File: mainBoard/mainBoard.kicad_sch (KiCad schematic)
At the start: 17 parts, among them J1 Conn_01x04, J2 Conn_01x04, J6 Conn_01x07, J7 Conn_01x07

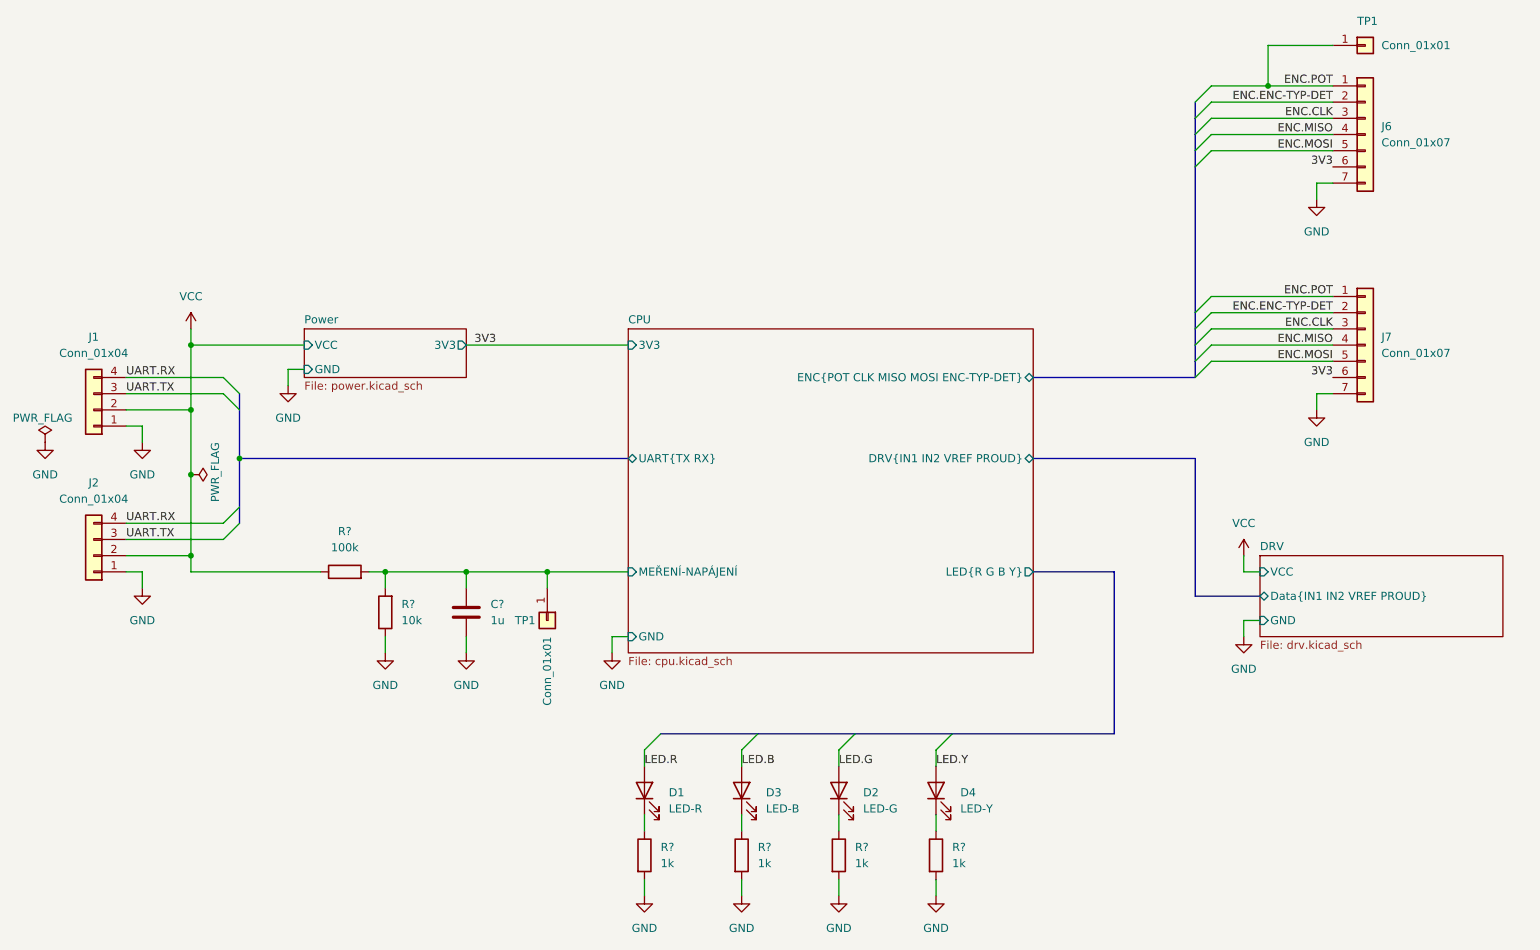
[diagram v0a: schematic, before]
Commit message: drobeček
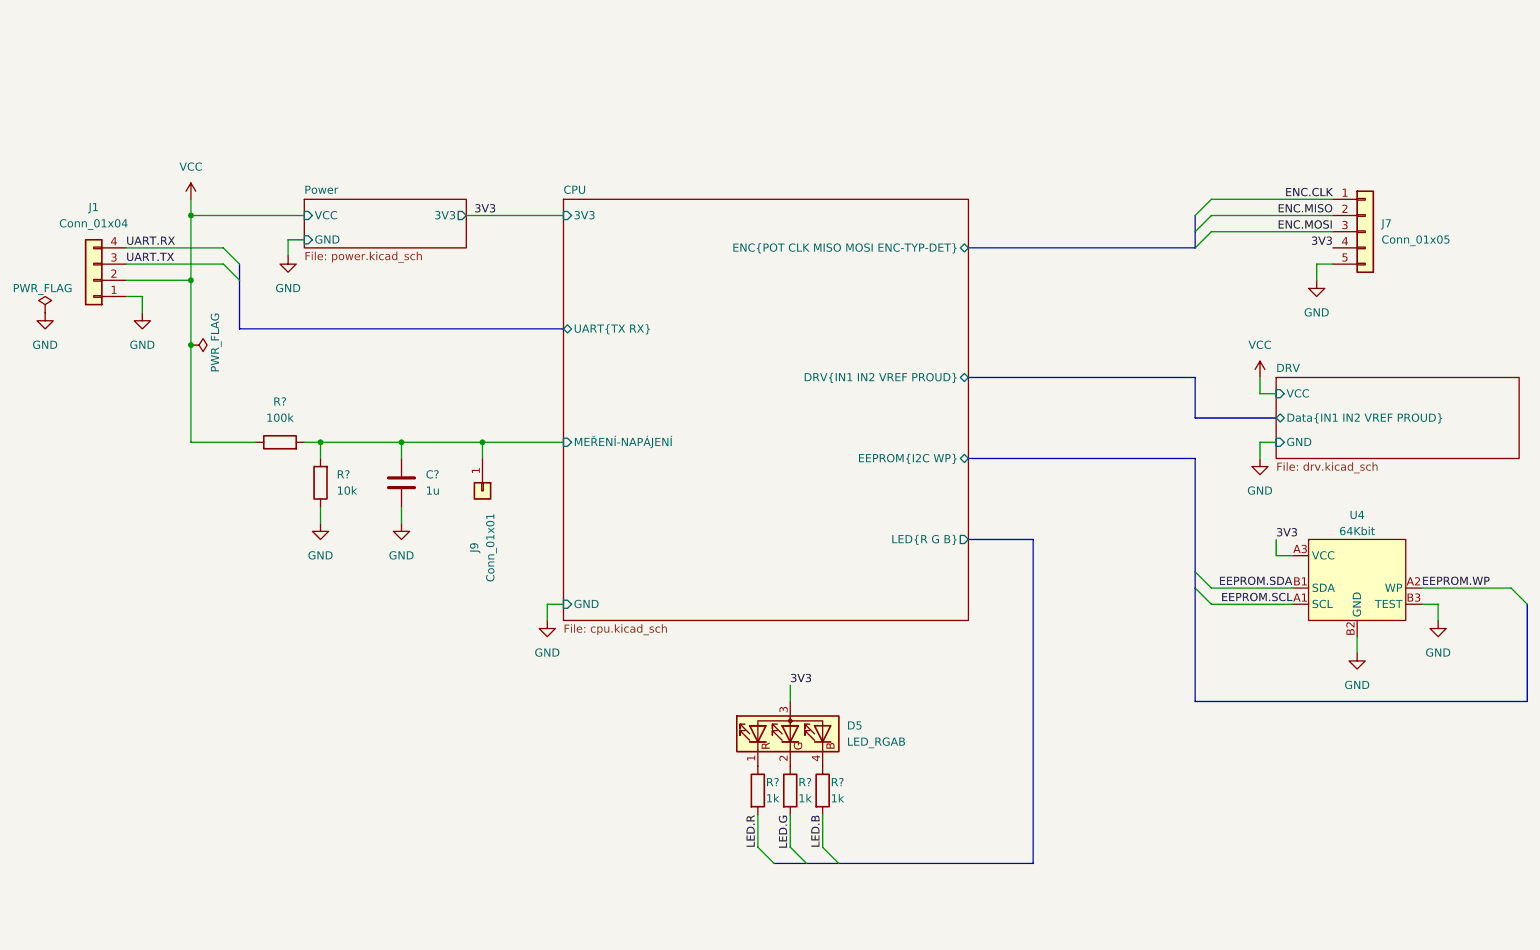
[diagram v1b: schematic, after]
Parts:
- removed D1: LED-R, LED_SMD:LED_0603_1608Metric, symbol Device:LED
- removed D2: LED-G, LED_SMD:LED_0603_1608Metric, symbol Device:LED
- removed D3: LED-B, LED_SMD:LED_0603_1608Metric, symbol Device:LED
- removed D4: LED-Y, LED_SMD:LED_0603_1608Metric, symbol Device:LED
- removed J2: Conn_01x04, Connector_JST:JST_PH_B4B-PH-K_1x04_P2.00mm_Vertical, symbol Connector_Generic:Conn_01x04
- removed J6: Conn_01x07, Connector_JST:JST_PH_B7B-PH-K_1x07_P2.00mm_Vertical, symbol Connector_Generic:Conn_01x07
- removed J7: Conn_01x07, Connector_PinHeader_1.27mm:PinHeader_1x07_P1.27mm_Vertical, symbol Connector_Generic:Conn_01x07
- removed R?: 1k, Capacitor_SMD:C_0402_1005Metric, symbol Device:R
- removed TP1 (x2): Conn_01x01, Connector_Pin:Pin_D1.0mm_L10.0mm, symbol Connector_Generic:Conn_01x01
- added D5: LED_RGAB, LED_SMD:LED_LiteOn_LTST-C19HE1WT, symbol Device:LED_RGAB
- added J7: Conn_01x05, Connector_PinHeader_2.00mm:PinHeader_1x05_P2.00mm_Vertical, symbol Connector_Generic:Conn_01x05
- added J9: Conn_01x01, RKL-Connectors:YZ157015035P-01-contact_pad, symbol Connector_Generic:Conn_01x01
- added U4: 64Kbit, RKL-StandardPackages:XFBGA-6, symbol RKL-Memory:BRCC064GWZ-3E2
- R?: footprint Capacitor_SMD:C_0402_1005Metric -> Resistor_SMD:R_0201_0603Metric; LCSC C25744 -> C473048
- R? (x3): footprint Capacitor_SMD:C_0402_1005Metric -> Capacitor_SMD:C_0201_0603Metric; LCSC C852624 -> C138165
- R?: footprint Capacitor_SMD:C_0402_1005Metric -> Resistor_SMD:R_0201_0603Metric; LCSC C25741 -> C320497
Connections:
- net 3V3: now also D5.3 (A), J7.4 (Pin_4), U4.A3 (VCC)
- net CPU/MEŘENÍ-NAPÁJENÍ: now also J9.1 (Pin_1)
- net ENC.CLK: now also J7.1 (Pin_1)
- net ENC.MISO: now also J7.2 (Pin_2)
- net ENC.MOSI: now also J7.3 (Pin_3)
- net GND: now also J7.5 (Pin_5), U4.B2 (GND), U4.B3 (TEST); no longer R?.2, R?.2, R?.2
- net LED.B: now also R?.2
- net LED.G: now also R?.2
- net LED.R: now also R?.2
- net at R?.1: now also D5.1 (RK)
- net at R?.1: now also D5.4 (BK)
- net at R?.1: now also D5.2 (GK)
- new net EEPROM.SCL: U4.A1 (SCL)
- new net EEPROM.SDA: U4.B1 (SDA)
- new net EEPROM.WP: U4.A2 (WP)
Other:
- sheet CPU ports: added EEPROM{I2C WP}, LED{R G B}; removed LED{R G B Y}
- moved on the sheet: C?, J1, R?

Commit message: Wpi
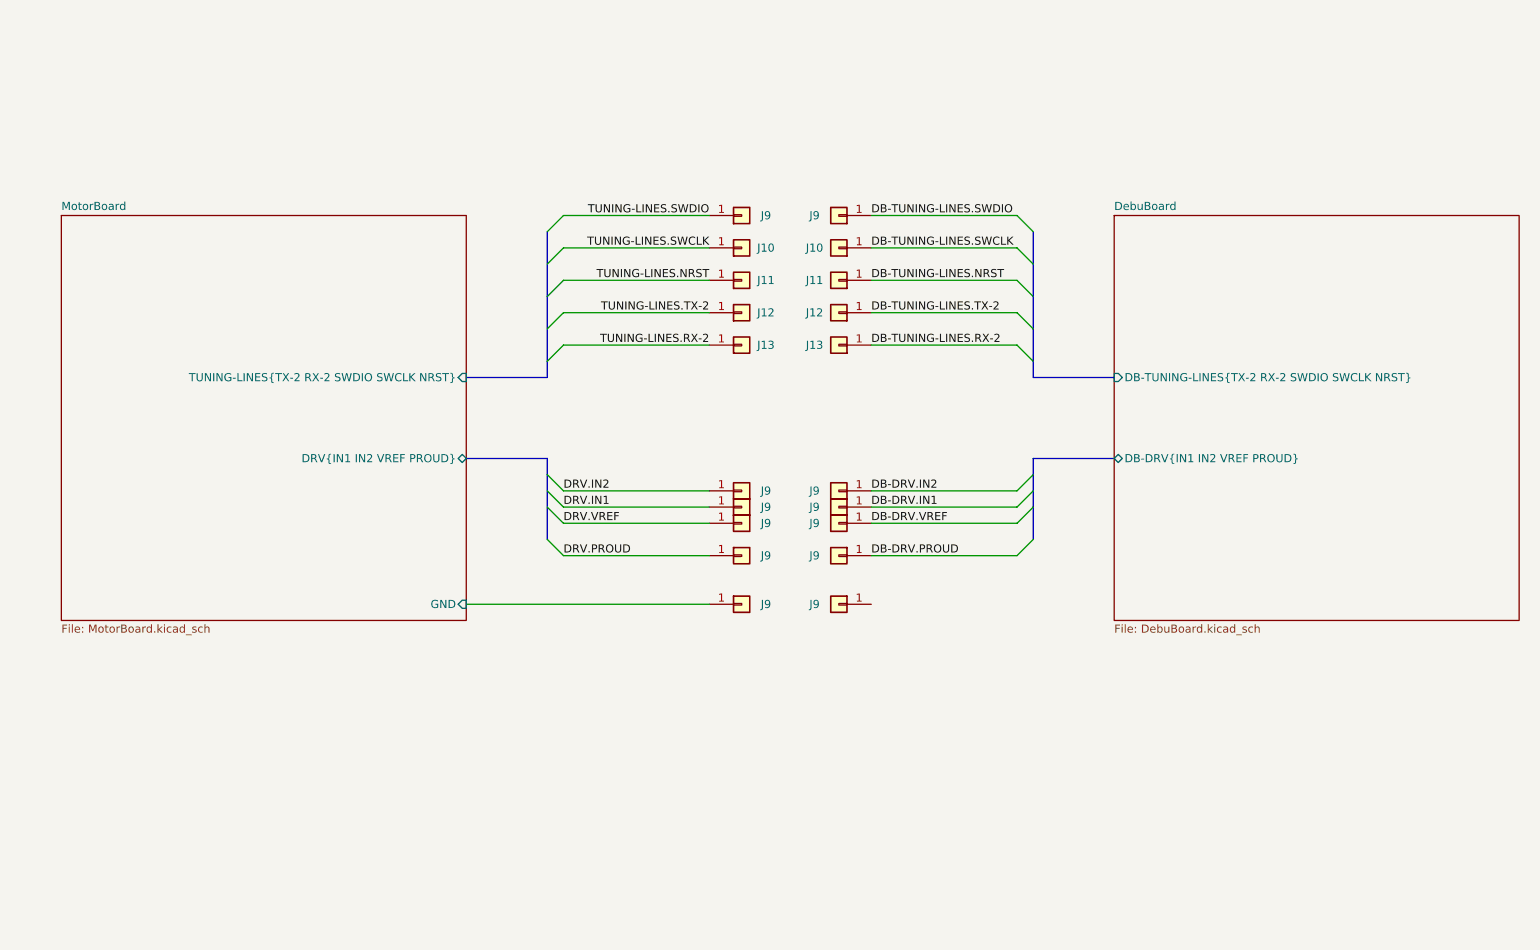
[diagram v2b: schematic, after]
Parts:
- removed C?: 1u, Capacitor_SMD:C_0402_1005Metric, symbol Device:C
- removed D5: LED_RGAB, LED_SMD:LED_LiteOn_LTST-C19HE1WT, symbol Device:LED_RGAB
- removed J1: Conn_01x04, Connector_JST:JST_PH_B4B-PH-K_1x04_P2.00mm_Vertical, symbol Connector_Generic:Conn_01x04
- removed J7: Conn_01x05, Connector_PinHeader_2.00mm:PinHeader_1x05_P2.00mm_Vertical, symbol Connector_Generic:Conn_01x05
- removed J9: Conn_01x01, RKL-Connectors:YZ157015035P-01-contact_pad, symbol Connector_Generic:Conn_01x01
- removed R?: 10k, Resistor_SMD:R_0201_0603Metric, symbol Device:R
- removed R? (x3): 1k, Capacitor_SMD:C_0201_0603Metric, symbol Device:R
- removed R?: 100k, Resistor_SMD:R_0201_0603Metric, symbol Device:R
- removed U4: 64Kbit, RKL-StandardPackages:XFBGA-6, symbol RKL-Memory:BRCC064GWZ-3E2
- added J10, J11, J12, J13, J9 (x6): Conn_01x01, RKL-Connectors:YZ157015035P-01, symbol Connector_Generic:Conn_01x01
- added J10, J11, J12, J13, J9 (x6): Conn_01x01, RKL-Connectors:YZ157015035P-01-contact_pad, symbol Connector_Generic:Conn_01x01
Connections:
- new net DB-DRV.IN1: J9.1 (Pin_1)
- new net DB-DRV.IN2: J9.1 (Pin_1)
- new net DB-DRV.PROUD: J9.1 (Pin_1)
- new net DB-DRV.VREF: J9.1 (Pin_1)
- new net DB-TUNING-LINES.NRST: J11.1 (Pin_1)
- new net DB-TUNING-LINES.RX-2: J13.1 (Pin_1)
- new net DB-TUNING-LINES.SWCLK: J10.1 (Pin_1)
- new net DB-TUNING-LINES.SWDIO: J9.1 (Pin_1)
- new net DB-TUNING-LINES.TX-2: J12.1 (Pin_1)
- new net DRV.IN1: J9.1 (Pin_1)
- new net DRV.IN2: J9.1 (Pin_1)
- new net DRV.PROUD: J9.1 (Pin_1)
- new net DRV.VREF: J9.1 (Pin_1)
- new net MotorBoard/GND: J9.1 (Pin_1)
- new net TUNING-LINES.NRST: J11.1 (Pin_1)
- new net TUNING-LINES.RX-2: J13.1 (Pin_1)
- new net TUNING-LINES.SWCLK: J10.1 (Pin_1)
- new net TUNING-LINES.SWDIO: J9.1 (Pin_1)
- new net TUNING-LINES.TX-2: J12.1 (Pin_1)
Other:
- removed sheet CPU
- removed sheet DRV
- removed sheet Power
- added sheet DebuBoard (DebuBoard.kicad_sch)
- added sheet MotorBoard (MotorBoard.kicad_sch)
